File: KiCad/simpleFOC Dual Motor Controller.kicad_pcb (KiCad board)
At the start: 4 copper layers, 50 x 50 mm, 69 parts, among them CN201 MR60-F, CN601 MR60-F, J101 Conn_01x04, Q301 AGM6014AP, Q303 AGM6014AP, Q401 AGM6014AP, Q403 AGM6014AP, Q501 AGM6014AP, Q503 AGM6014AP, Q701 AGM6014AP, Q703 AGM6014AP, Q801 AGM6014AP, Q803 AGM6014AP, Q901 AGM6014AP, Q903 AGM6014AP, SW101 TS-1088-AR02016, U101 STM32F103C8Tx, U102 XT60H-M, U201 DRV8323HRTAT, U601 DRV8323HRTAT

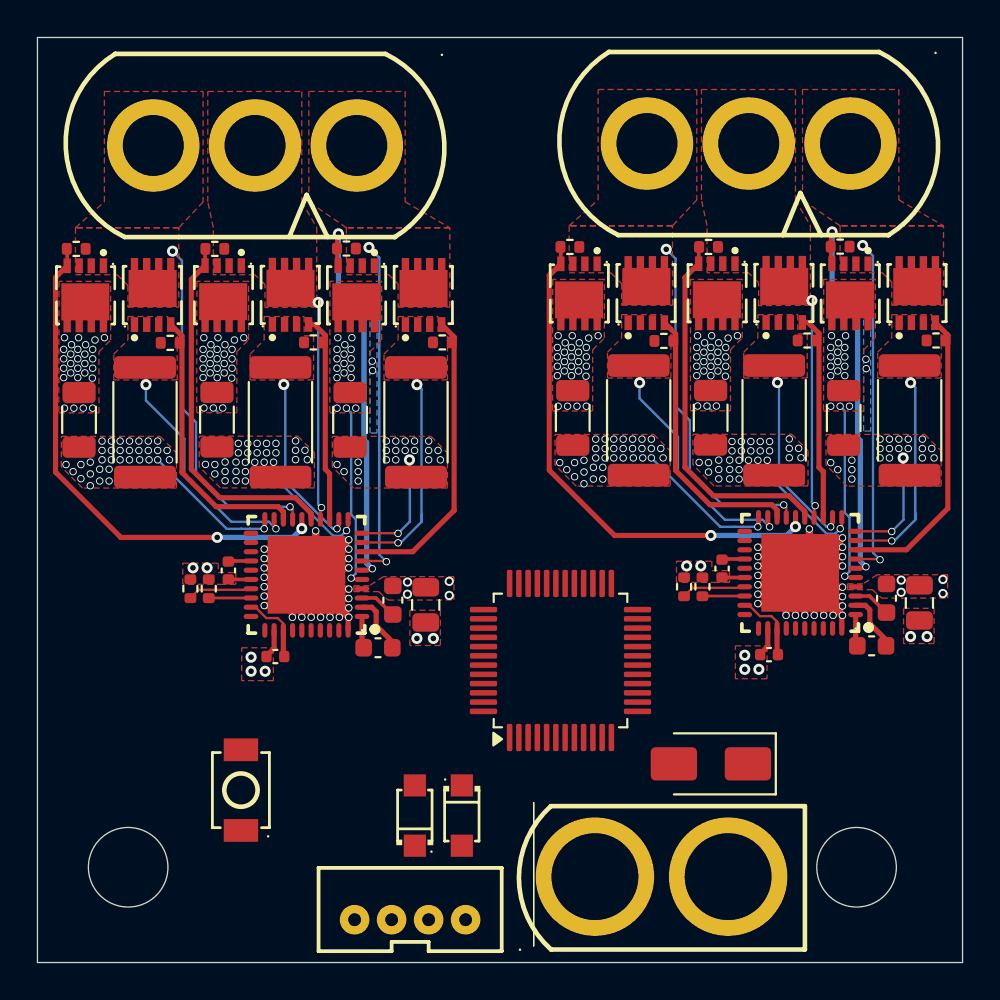
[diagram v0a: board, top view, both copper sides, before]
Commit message: condensed
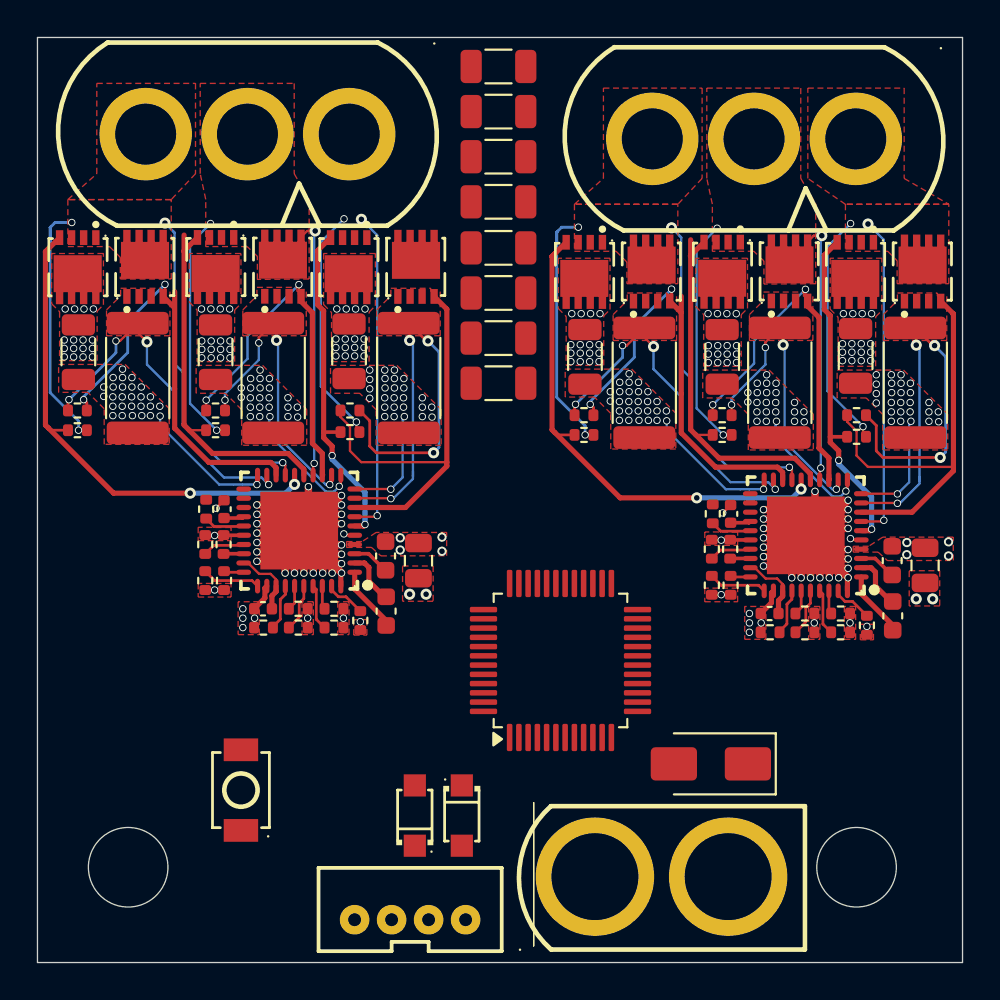
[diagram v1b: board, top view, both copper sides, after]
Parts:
- removed C601: 100n, Capacitor_SMD:C_0805_2012Metric
- removed C602: 1u, Capacitor_SMD:C_0603_1608Metric
- removed C603: 47n, Capacitor_SMD:C_0603_1608Metric
- removed C604: 1u, Capacitor_SMD:C_0402_1005Metric
- removed C605: 0.1u, Capacitor_SMD:C_0402_1005Metric
- removed C701, C801, C901: 10u, Capacitor_SMD:C_1206_3216Metric
- removed CN601: MR60-F, easyeda2kicad:CONN-TH_3P-P5.50_MR60-F
- removed NT601, NT602, NT603: NetTie_2, CustomNetTie:NetTie0.127mm
- removed Q701, Q703, Q801, Q803, Q901, Q903: AGM6014AP, easyeda2kicad:PDFN-8_L3.1-W3.0-P0.65-LS3.3-BL
- removed R601, R602: 75k, Resistor_SMD:R_0402_1005Metric
- removed R701, R702, R801, R802, R901, R902: 47k, Resistor_SMD:R_0402_1005Metric
- removed Rsns701, Rsns801, Rsns901: 0.001, Resistor_SMD:R_2512_6332Metric
- removed U601: DRV8323HRTAT, easyeda2kicad:WQFN-40_L6.0-W6.0-P0.50-TL-EP4.2
- added C108: 10u, Capacitor_SMD:C_1206_3216Metric, F.Cu at (116.8, 42.0)
- added C109: 10u, Capacitor_SMD:C_1206_3216Metric, F.Cu at (102.2, 42.0)
- added C110: 10u, Capacitor_SMD:C_1206_3216Metric, F.Cu at (109.6, 42.0)
- added C206: 100n, Capacitor_SMD:C_0805_2012Metric, F.Cu at (120.6, 53.3)
- added C207: 1u, Capacitor_SMD:C_0603_1608Metric, F.Cu at (118.8, 53.0)
- added C208: 47n, Capacitor_SMD:C_0603_1608Metric, F.Cu at (118.8, 56.0)
- added C209: 0.1u, Capacitor_SMD:C_0402_1005Metric, F.Cu at (110.1, 50.5)
- added C210: 1u, Capacitor_SMD:C_0402_1005Metric, F.Cu at (112.2, 55.9)
- added C401: 10u, Capacitor_SMD:C_1206_3216Metric, F.Cu at (124.9, 31.4)
- added C401: 10u, Capacitor_SMD:C_1206_3216Metric, F.Cu at (124.9, 29.0)
- added C401: 10u, Capacitor_SMD:C_1206_3216Metric, F.Cu at (124.9, 38.8)
- added C401: 10u, Capacitor_SMD:C_1206_3216Metric, F.Cu at (124.9, 43.7)
- added C401: 10u, Capacitor_SMD:C_1206_3216Metric, F.Cu at (124.9, 26.6)
- added C401: 10u, Capacitor_SMD:C_1206_3216Metric, F.Cu at (124.9, 33.9)
- added C401: 10u, Capacitor_SMD:C_1206_3216Metric, F.Cu at (124.9, 41.2)
- added C401: 10u, Capacitor_SMD:C_1206_3216Metric, F.Cu at (124.9, 36.4)
- added CN202: MR60-F, easyeda2kicad:CONN-TH_3P-P5.50_MR60-F, F.Cu at (111.3, 30.2)
- added NT204: NetTie_2, CustomNetTie:NetTie0.127mm, B.Cu at (119.7, 46.3)
- added NT205: NetTie_2, CustomNetTie:NetTie0.127mm, B.Cu at (112.5, 46.0)
- added NT206: NetTie_2, CustomNetTie:NetTie0.127mm, B.Cu at (110.8, 49.2)
- added Q101: AGM6014AP, easyeda2kicad:PDFN-8_L3.1-W3.0-P0.65-LS3.3-BL, F.Cu at (116.8, 37.4)
- added Q102: AGM6014AP, easyeda2kicad:PDFN-8_L3.1-W3.0-P0.65-LS3.3-BL, F.Cu at (109.6, 37.4)
- added Q103: AGM6014AP, easyeda2kicad:PDFN-8_L3.1-W3.0-P0.65-LS3.3-BL, F.Cu at (102.2, 37.4)
- added Q104: AGM6014AP, easyeda2kicad:PDFN-8_L3.1-W3.0-P0.65-LS3.3-BL, F.Cu at (120.5, 37.4)
- added Q105: AGM6014AP, easyeda2kicad:PDFN-8_L3.1-W3.0-P0.65-LS3.3-BL, F.Cu at (113.3, 37.4)
- added Q106: AGM6014AP, easyeda2kicad:PDFN-8_L3.1-W3.0-P0.65-LS3.3-BL, F.Cu at (105.8, 37.4)
- added R101: 47k, Resistor_SMD:R_0402_1005Metric, F.Cu at (116.9, 46.3)
- added R102: 47k, Resistor_SMD:R_0402_1005Metric, F.Cu at (109.6, 46.2)
- added R103: 47k, Resistor_SMD:R_0402_1005Metric, F.Cu at (102.2, 46.2)
- added R104: 47k, Resistor_SMD:R_0402_1005Metric, F.Cu at (116.9, 45.2)
- added R105: 47k, Resistor_SMD:R_0402_1005Metric, F.Cu at (109.6, 45.2)
- added R106: 47k, Resistor_SMD:R_0402_1005Metric, F.Cu at (102.2, 45.2)
- added R203: 100k, Resistor_SMD:R_0402_1005Metric, F.Cu at (139.6, 57.1)
- added R204: 100k, Resistor_SMD:R_0402_1005Metric, F.Cu at (141.5, 56.1)
- added R205: 100k, Resistor_SMD:R_0402_1005Metric, F.Cu at (141.5, 57.1)
- added R206: 100k, Resistor_SMD:R_0402_1005Metric, F.Cu at (143.4, 57.1)
- added R207: 100k, Resistor_SMD:R_0402_1005Metric, F.Cu at (143.4, 56.1)
- added R208: 100k, Resistor_SMD:R_0402_1005Metric, F.Cu at (144.8, 56.8)
- added R209: 100k, Resistor_SMD:R_0402_1005Metric, F.Cu at (137.5, 54.6)
- added R210: 100k, Resistor_SMD:R_0402_1005Metric, F.Cu at (136.4, 54.6)
- added R211: 100k, Resistor_SMD:R_0402_1005Metric, F.Cu at (136.5, 50.7)
- added R212: 75k, Resistor_SMD:R_0402_1005Metric, F.Cu at (110.1, 52.4)
- added R213: 75k, Resistor_SMD:R_0402_1005Metric, F.Cu at (109.1, 52.4)
- added R214: 100k, Resistor_SMD:R_0402_1005Metric, F.Cu at (112.2, 56.9)
- added R215: 100k, Resistor_SMD:R_0402_1005Metric, F.Cu at (114.1, 55.9)
- added R216: 100k, Resistor_SMD:R_0402_1005Metric, F.Cu at (114.1, 56.9)
- added R217: 100k, Resistor_SMD:R_0402_1005Metric, F.Cu at (116.0, 56.9)
- added R218: 100k, Resistor_SMD:R_0402_1005Metric, F.Cu at (116.0, 55.9)
- added R219: 100k, Resistor_SMD:R_0402_1005Metric, F.Cu at (117.4, 56.5)
- added R220: 100k, Resistor_SMD:R_0402_1005Metric, F.Cu at (110.1, 54.4)
- added R221: 100k, Resistor_SMD:R_0402_1005Metric, F.Cu at (109.1, 54.4)
- added R222: 100k, Resistor_SMD:R_0402_1005Metric, F.Cu at (109.1, 50.5)
- added Rsns101: 0.001, Resistor_SMD:R_2512_6332Metric, F.Cu at (120.1, 43.4)
- added Rsns102: 0.001, Resistor_SMD:R_2512_6332Metric, F.Cu at (112.7, 43.4)
- added Rsns103: 0.001, Resistor_SMD:R_2512_6332Metric, F.Cu at (105.4, 43.4)
- added U202: DRV8323HRTAT, easyeda2kicad:WQFN-40_L6.0-W6.0-P0.50-TL-EP4.2, F.Cu at (114.1, 51.7)
- moved R302 10.3 mm to (144.3, 46.6)
- moved R502 10.2 mm to (129.5, 46.5)
- moved R402 10.2 mm to (137.0, 46.5)
- moved R401 6.11 mm to (137.0, 45.4), turned to 0 degrees
- moved R301 5.90 mm to (144.3, 45.4), turned to 0 degrees
- moved R501 5.90 mm to (129.5, 45.4)
- moved C301 3.41 mm to (144.2, 42.2)
- moved C401 3.37 mm to (129.6, 42.3)
- moved C501 3.35 mm to (137.0, 42.3)
- moved C205 2.99 mm to (137.5, 50.7), turned to 90 degrees
- moved R201 2.53 mm to (136.4, 52.7)
- moved R202 2.53 mm to (137.4, 52.7)
- moved C204 2.22 mm to (139.6, 56.1)
- moved NT202 2.07 mm to (139.9, 46.2)
- moved C201 2.05 mm to (148.0, 53.5)
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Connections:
- U101 pad 25: unconnected-(U101-PB12-Pad25) -> /FAULT1
- U101 pad 3: unconnected-(U101-PC14-Pad3) -> /FAULT2
- U101 pad 45: unconnected-(U101-PB8-Pad45) -> /EN1
- U101 pad 46: unconnected-(U101-PB9-Pad46) -> /CAL1
- U101 pad 5: unconnected-(U101-PD0-Pad5) -> /EN2
- U101 pad 6: unconnected-(U101-PD1-Pad6) -> /CAL2
- U201 pad 25: /Motor Driver 1/FAULT -> /Motor Driver 1/~{FAULT}
- U201 pad 30: /Motor Driver 1/EN -> /EN1
- U201 pad 31: /Motor Driver 1/CAL -> /CAL1
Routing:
- net /Motor Driver 1/Motor_VIN: track 84.1 -> 0.00 mm, vias 22 -> 0
- net GND: track 74.7 -> 146.8 mm, vias 293 -> 220
- net /Motor Driver 1/Pole 2/PoleOut: track 13.6 -> 28.3 mm, vias 2 -> 4
- net /Motor Driver 2/Pole 2/PoleOut: track 13.6 -> 28.3 mm, vias 2 -> 4
- net /Motor Driver 2/Pole 3/PoleOut: track 19.1 -> 32.7 mm, vias 2 -> 4
- net /Motor Driver 1/Pole 3/PoleOut: track 19.1 -> 32.7 mm, vias 2 -> 4
- net /Motor Driver 1/Pole 1/SP: track 12.6 -> 25.9 mm, vias 2 -> 4
- net /Motor Driver 2/Pole 1/SP: track 12.6 -> 25.9 mm, vias 2 -> 4
- net /Motor Driver 2/Pole 1/PoleOut: track 18.7 -> 30.6 mm, vias 2 -> 4
- net /Motor Driver 1/Pole 1/PoleOut: track 18.7 -> 30.6 mm, vias 2 -> 4
- net /Motor Driver 1/Pole 3/GL: track 15.0 -> 24.5 mm, vias 0 -> 2
- net /Motor Driver 2/Pole 3/GL: track 15.0 -> 24.5 mm, vias 0 -> 2
- net M+: track 10.1 -> 1.23 mm, vias 71 -> 106
- net /Motor Driver 1/Pole 2/GL: track 11.2 -> 19.7 mm, vias 0 -> 2
- net /Motor Driver 2/Pole 2/GL: track 11.2 -> 19.7 mm, vias 0 -> 2
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- removed copper zone on F.Cu, net /Motor Driver 2/Pole 1/PoleOut
- removed copper zone on B.Cu, net GND
